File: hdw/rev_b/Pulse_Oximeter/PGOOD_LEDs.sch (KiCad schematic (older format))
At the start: 18 parts, among them U1801 TPS71530, U1802 74LVC1G06, U1803 74LVC1G06, U1805 74LVC1G06, U1806 74LVC1G06

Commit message: changed PGOOD LED drivers
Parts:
- removed C1801: 0.1uF, Capacitors_SMD:C_0402, symbol Custom_Library:C_Custom
- removed C1802: 10uF, Capacitors_SMD:C_0402, symbol Custom_Library:C_Custom
- removed U1801: TPS71530, Package_TO_SOT_SMD:SOT-353_SC-70-5, symbol Regulator_Linear:TPS71530__SC70
- removed U1802, U1803, U1805, U1806: 74LVC1G06, TO_SOT_Packages_SMD:SOT-353_SC-70-5, symbol Custom_Library:74LVC1G06_Power
- added R?: 10k, Resistors_SMD:R_0402, symbol Custom_Library:R_Custom
- added U? (x4): 74LVC1G97, Package_TO_SOT_SMD:SOT-363_SC-70-6, symbol Custom_Library:74LVC1G97_Power_AND
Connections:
- net labels added: PGOOD_LED_EN
- net labels removed: +12V
- wire segments 17 -> 11

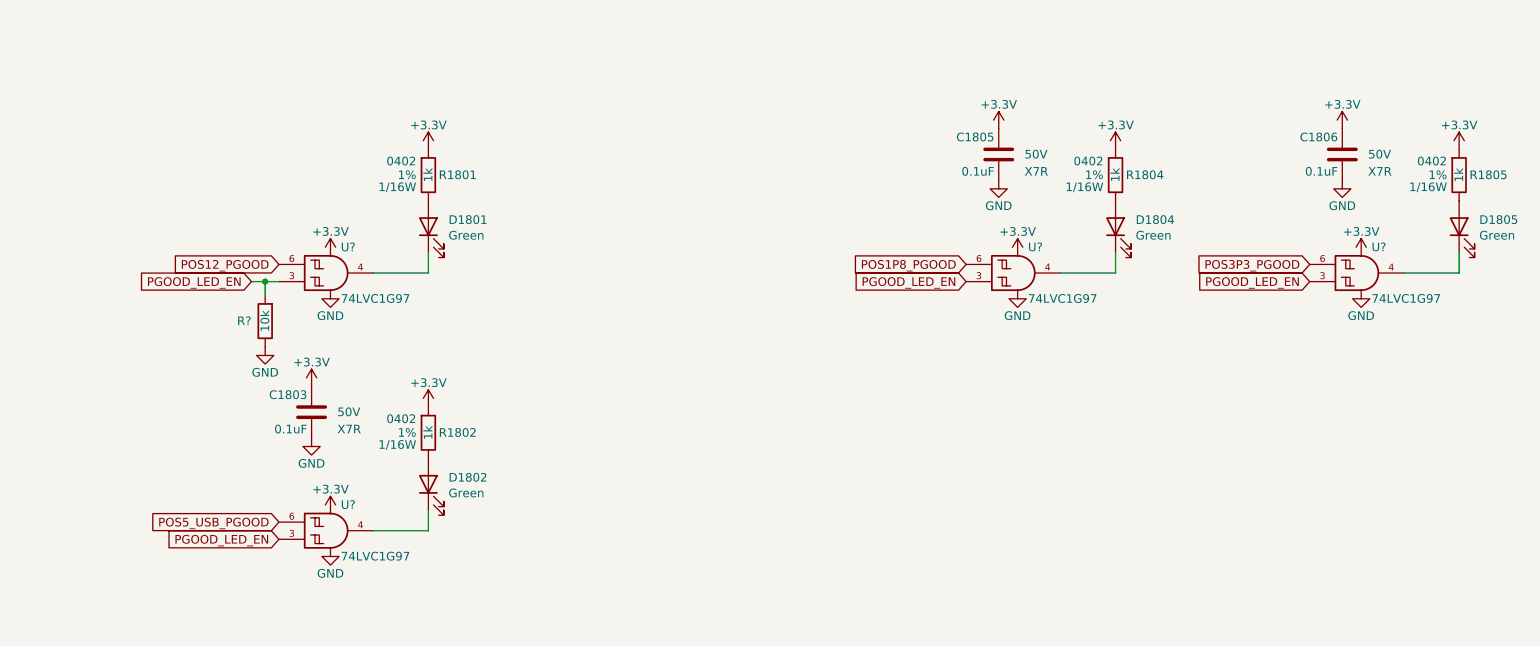
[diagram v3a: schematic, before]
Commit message: changed all passives to 0402, cleared digikey pns
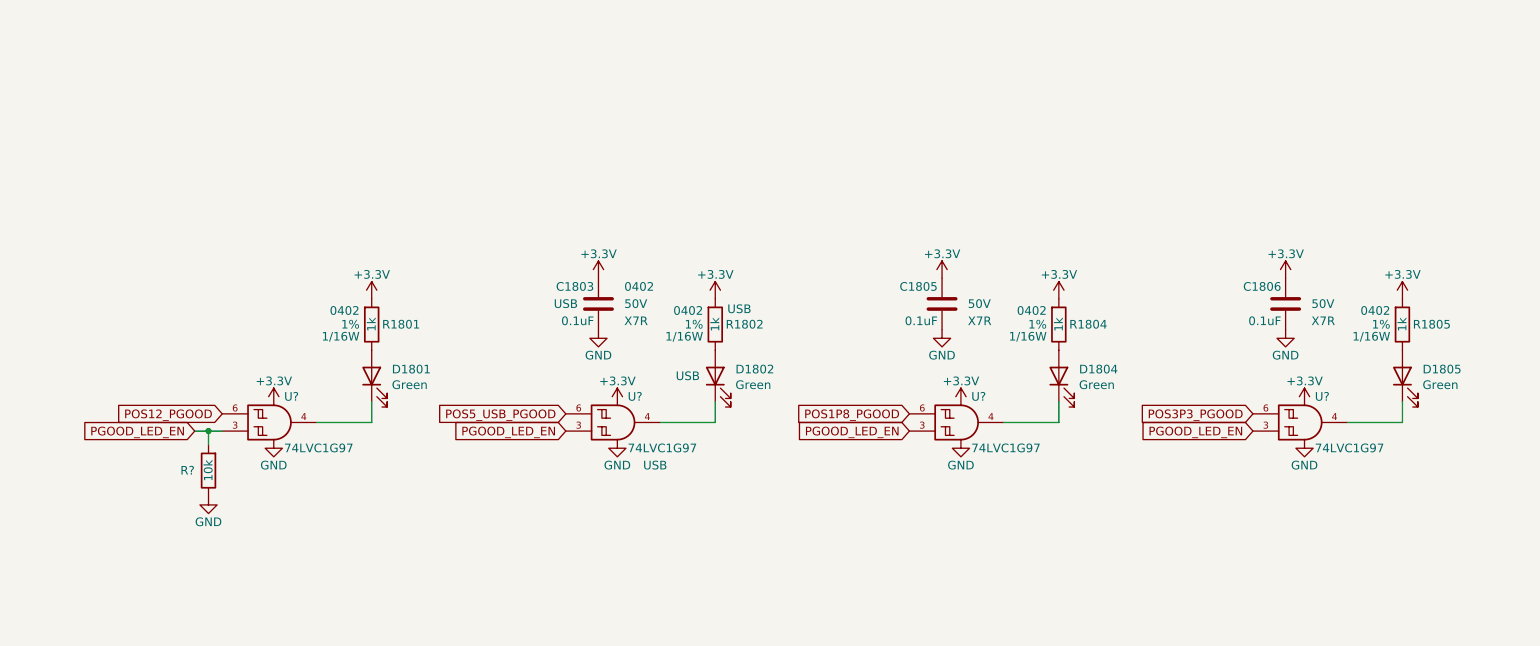
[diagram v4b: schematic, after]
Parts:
- C1803: footprint Capacitors_SMD:C_0402 -> (none); Configuration (none) -> USB; Digi-Key PN 490-10701-1-ND -> (none); display_footprint (none) -> 0402
- C1805, C1806: Digi-Key PN 490-10701-1-ND -> (none)
- D1802, U?: Configuration (none) -> USB
- R1801, R1804, R1805: Digi-Key PN 541-1.00KLCT-ND -> (none)
- R1802: Configuration (none) -> USB; Digi-Key PN 541-1.00KLCT-ND -> (none)
- R?: Digi-Key PN RMCF0402FT10K0CT-ND -> (none)
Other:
- moved on the sheet: C1803, C1805, C1806, D1801, D1802, D1804, D1805, R1801, R1802, R1804, R1805, R?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
